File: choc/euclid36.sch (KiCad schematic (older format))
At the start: 130 parts, among them SW10 SW_PUSH, SW11 SW_PUSH, SW12 SW_PUSH, SW14 SW_PUSH, SW15 SW_PUSH, SW16 SW_PUSH, SW17 SW_PUSH, SW18 SW_PUSH, SW19 SW_PUSH, SW2 SW_PUSH, SW20 SW_PUSH, SW21 SW_PUSH, SW22 SW_PUSH, SW23 SW_PUSH, SW25 SW_PUSH, SW26 SW_PUSH, SW27 SW_PUSH, SW28 SW_PUSH, SW29 SW_PUSH, SW3 SW_PUSH, SW31 SW_PUSH, SW32 SW_PUSH, SW33 SW_PUSH, SW34 SW_PUSH, SW35 SW_PUSH, SW37 SW_PUSH, SW38 SW_PUSH, SW39 SW_PUSH, SW4 SW_PUSH, SW40 SW_PUSH, SW41 SW_PUSH, SW42 SW_PUSH, SW5 SW_PUSH, SW6 SW_PUSH, SW8 SW_PUSH, SW9 SW_PUSH, U1 USBLC6-2SC6, U2 ATmega32U4-AU, Y1 XTAL

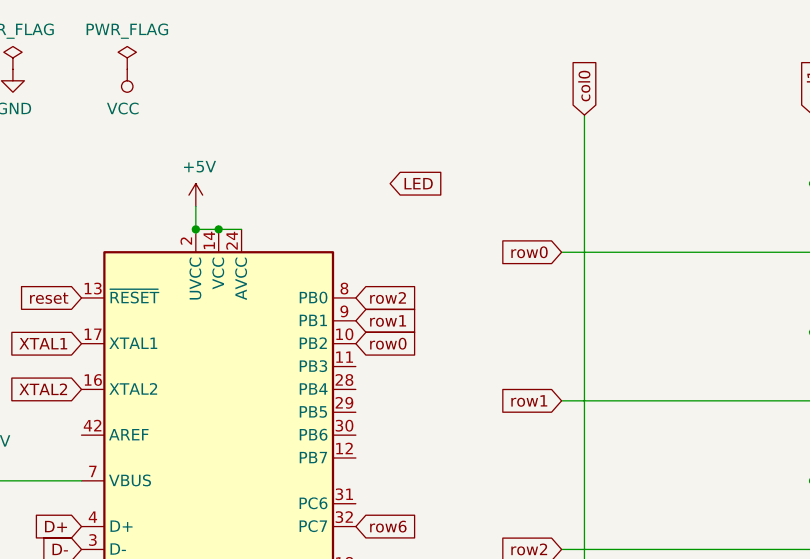
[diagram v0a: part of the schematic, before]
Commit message: latest low pro choc keyboard
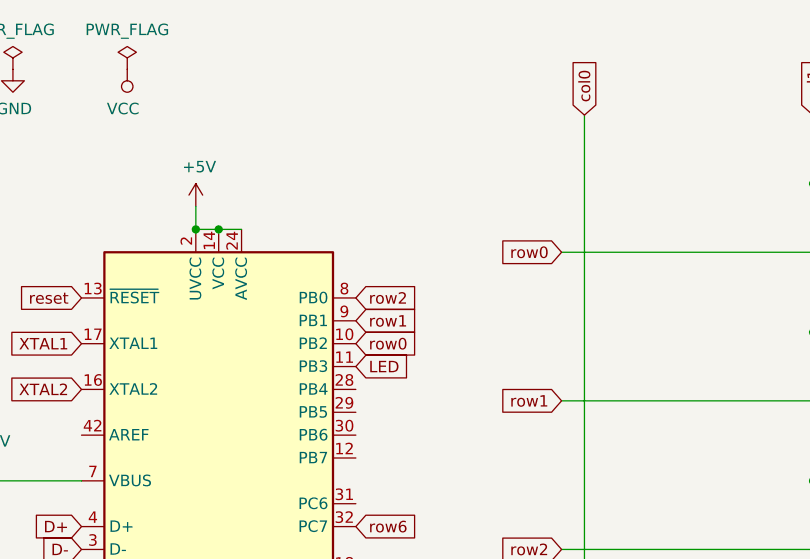
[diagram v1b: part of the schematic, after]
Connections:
- net LED: now also U2.11 (PB3)
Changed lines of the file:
@@
 Text GLabel 1100 1850 0    50   Input ~ 0
 reset
-Text GLabel 2450 1350 2    50   Input ~ 0
+Text GLabel 2300 2150 2    50   Input ~ 0
 LED
 $Comp
